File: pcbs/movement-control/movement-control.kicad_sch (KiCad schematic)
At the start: 27 parts

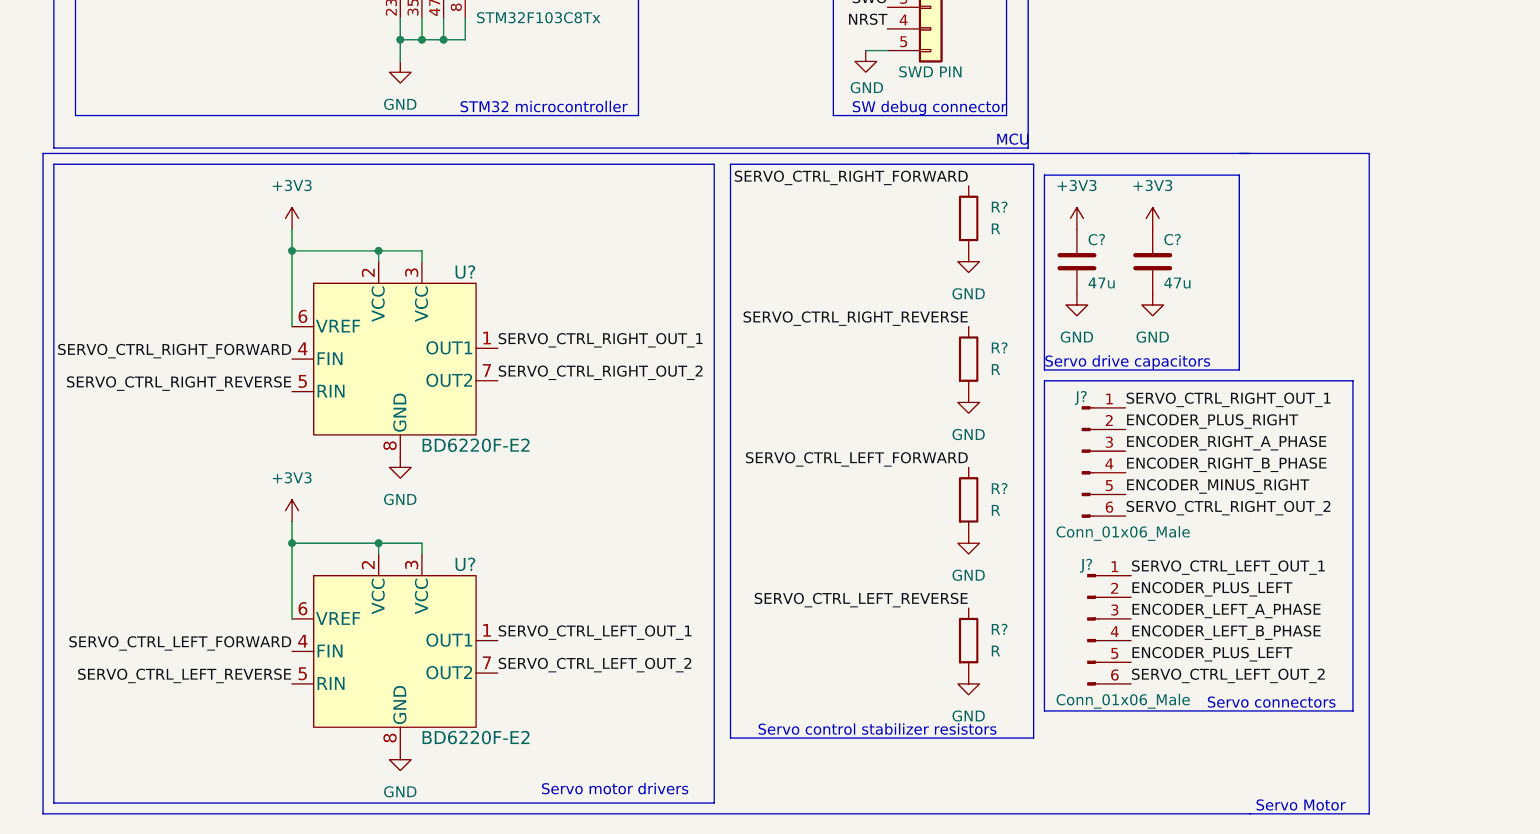
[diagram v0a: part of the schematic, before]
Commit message: Reposition schematic elements
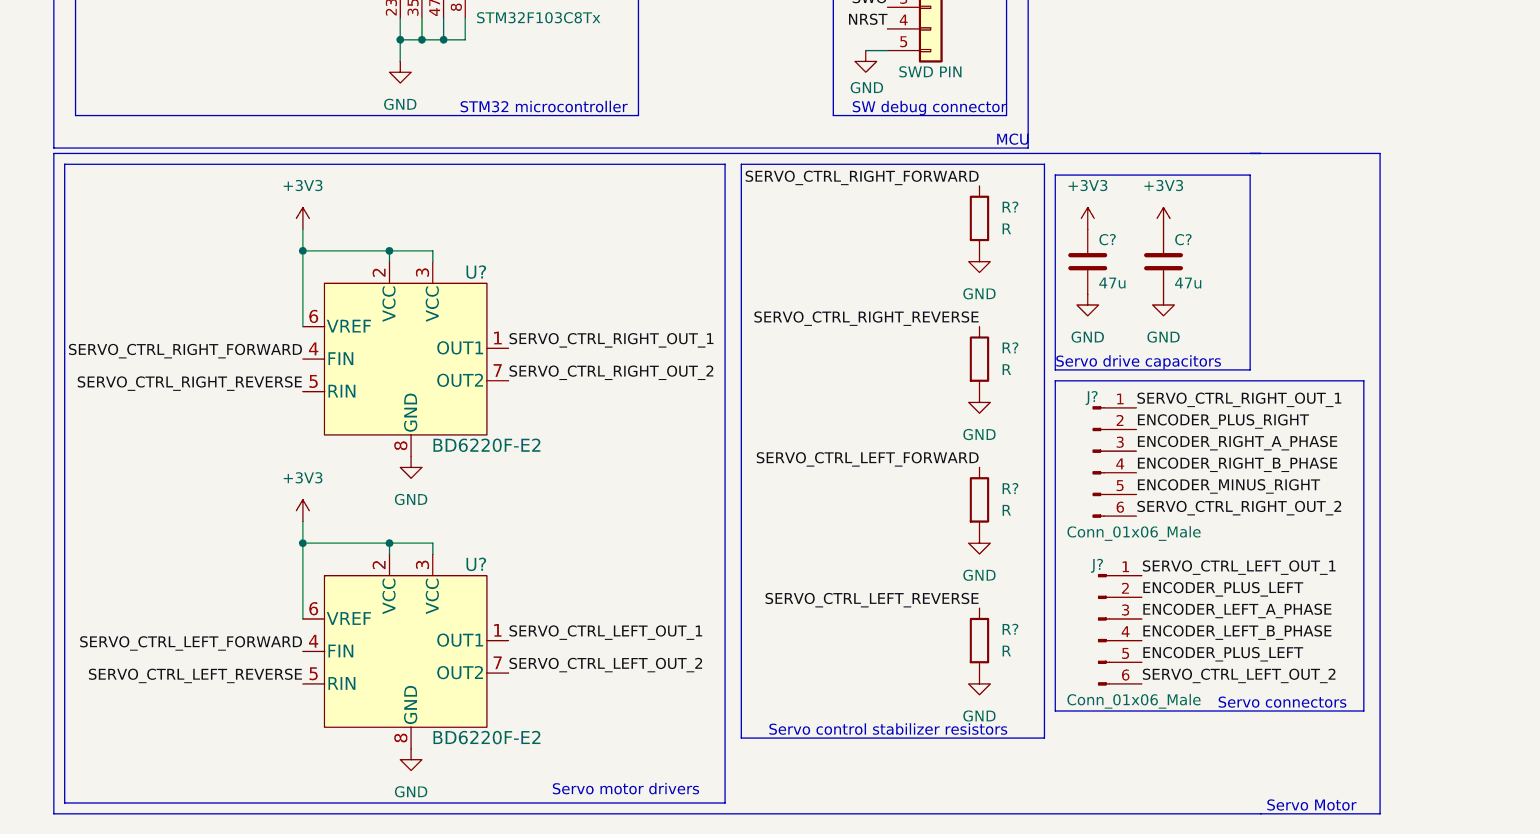
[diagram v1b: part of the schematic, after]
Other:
- moved on the sheet: C?, J?, R?, U?
